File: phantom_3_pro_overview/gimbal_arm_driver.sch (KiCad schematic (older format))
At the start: 0 parts

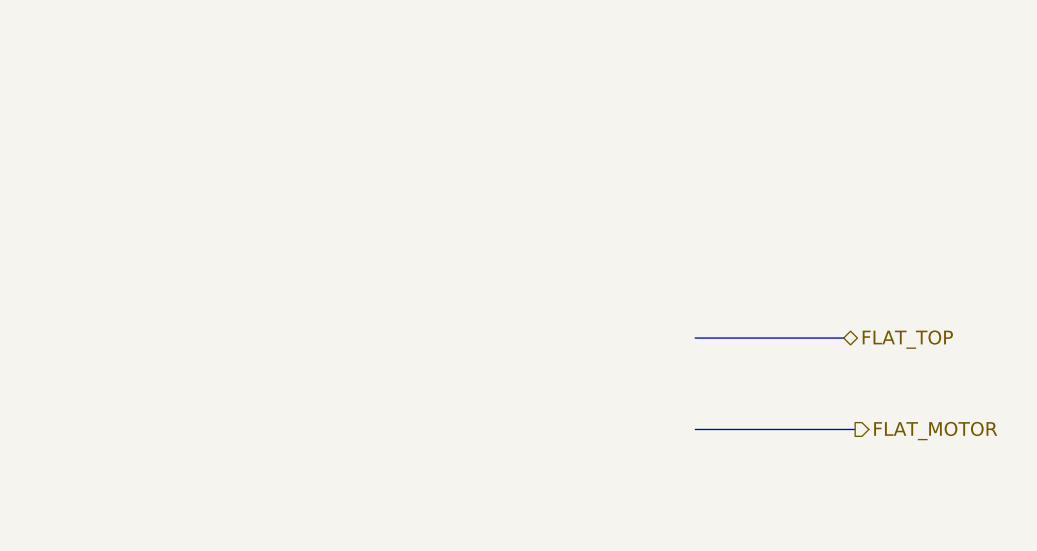
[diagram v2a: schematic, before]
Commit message: Overview: Work on camera and gimbal.
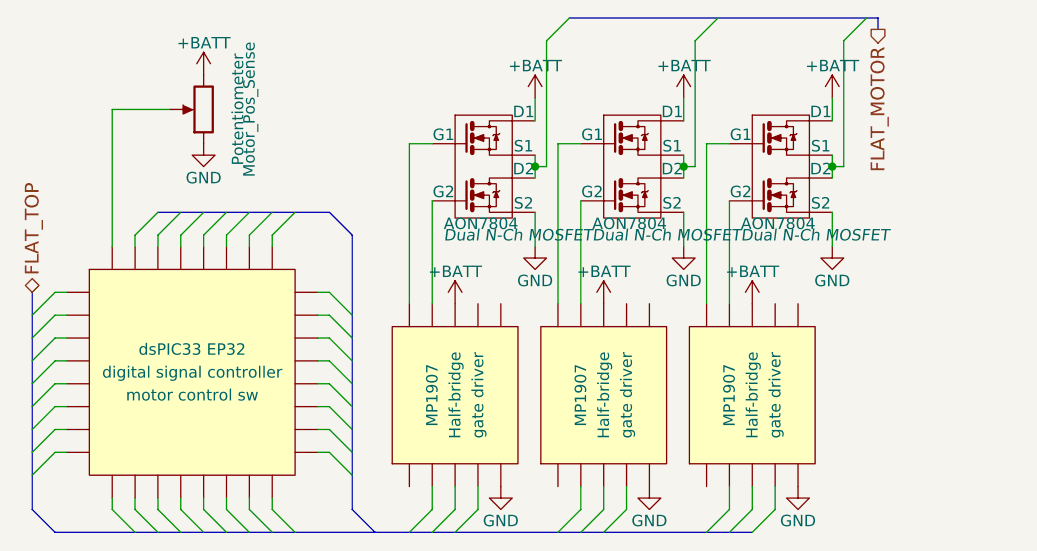
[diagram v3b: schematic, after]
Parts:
- added Q? (x3): AON7804, Dual N-Ch MOSFET, symbol AON7804-align1
- added RV?: Potentiometer, Motor_Pos_Sense, symbol POT
- added U?: dsPIC33 EP32, motor control sw, symbol IC_PQFP32
- added U? (x3): MP1907, Half-bridge, symbol IC_DIL10
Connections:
- new net: RV?.2, U?.32
- new net: Q?.1 (G1), U?.5 (x3)
- new net: Q?.2 (S1), Q?.4 (D2) (x3)
- new net: Q?.5 (G2), U?.4 (x3)
- new net +BATT: Q?.8 (D1), Q?.8 (D1), Q?.8 (D1), RV?.3, U?.3, U?.3, U?.3
- new net GND: Q?.6 (S2), Q?.6 (S2), Q?.6 (S2), RV?.1, U?.10, U?.10, U?.10
